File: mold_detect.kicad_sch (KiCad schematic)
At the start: 39 parts, among them J1 USB_C_Receptacle_USB2.0_14P, U1 SHT30-DIS, U2 TPL5010, U3 FT230XS, U4 W25Q128JVS, U5 ATmega328P-P, Y1 4MHz

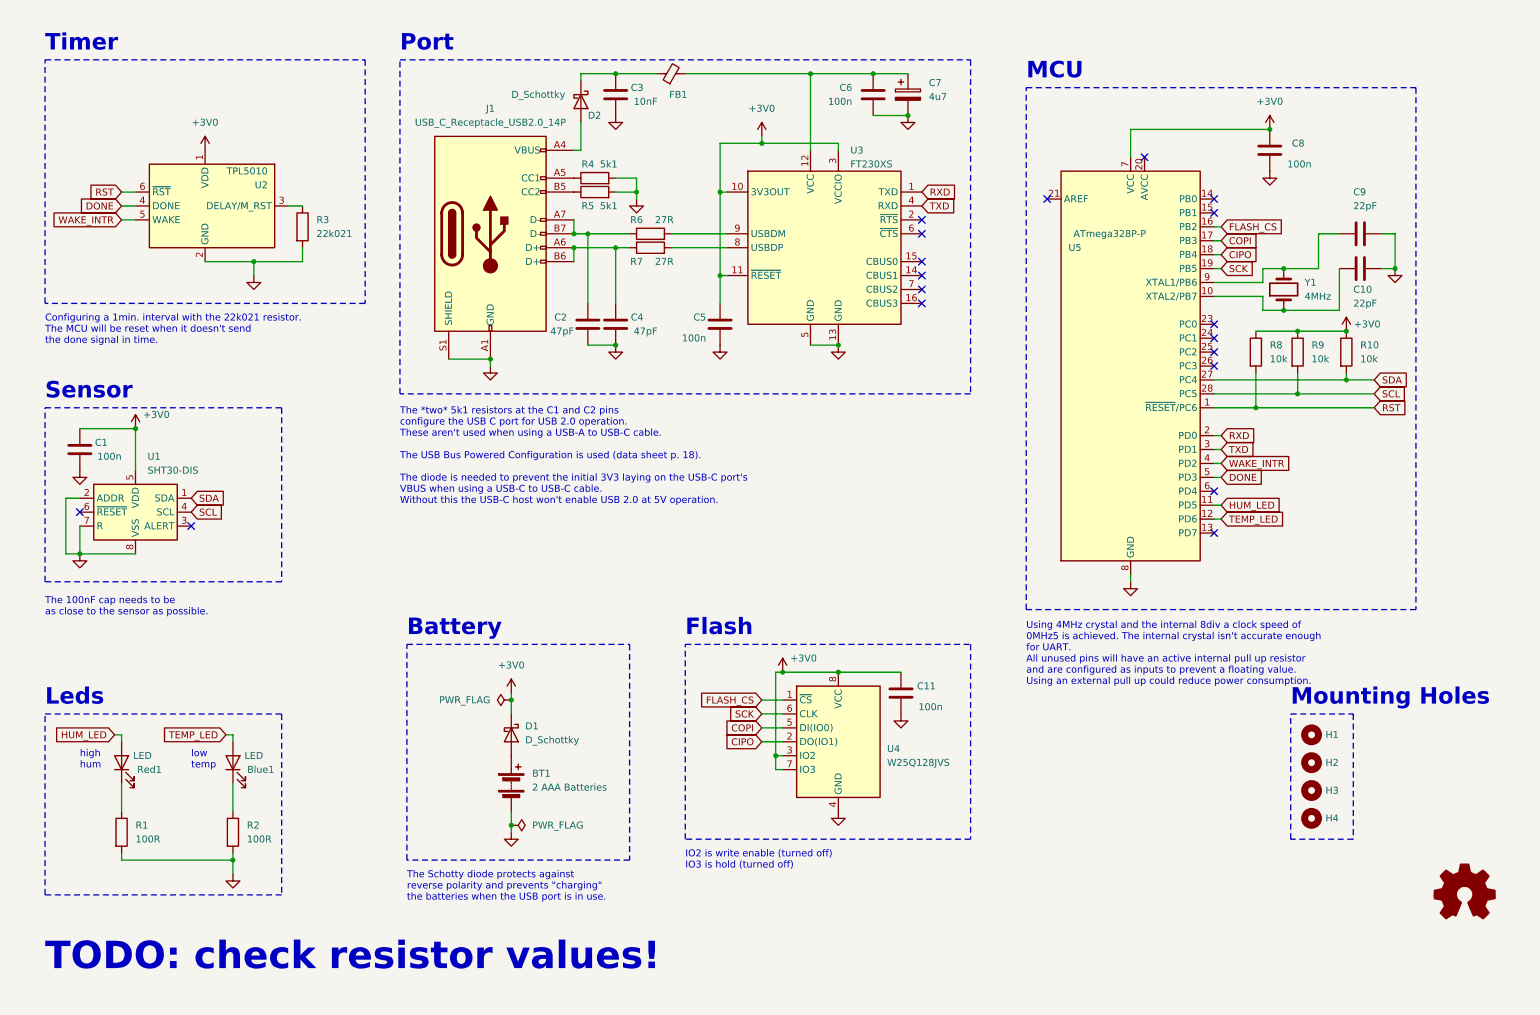
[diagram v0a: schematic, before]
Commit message: tpl5010 works!
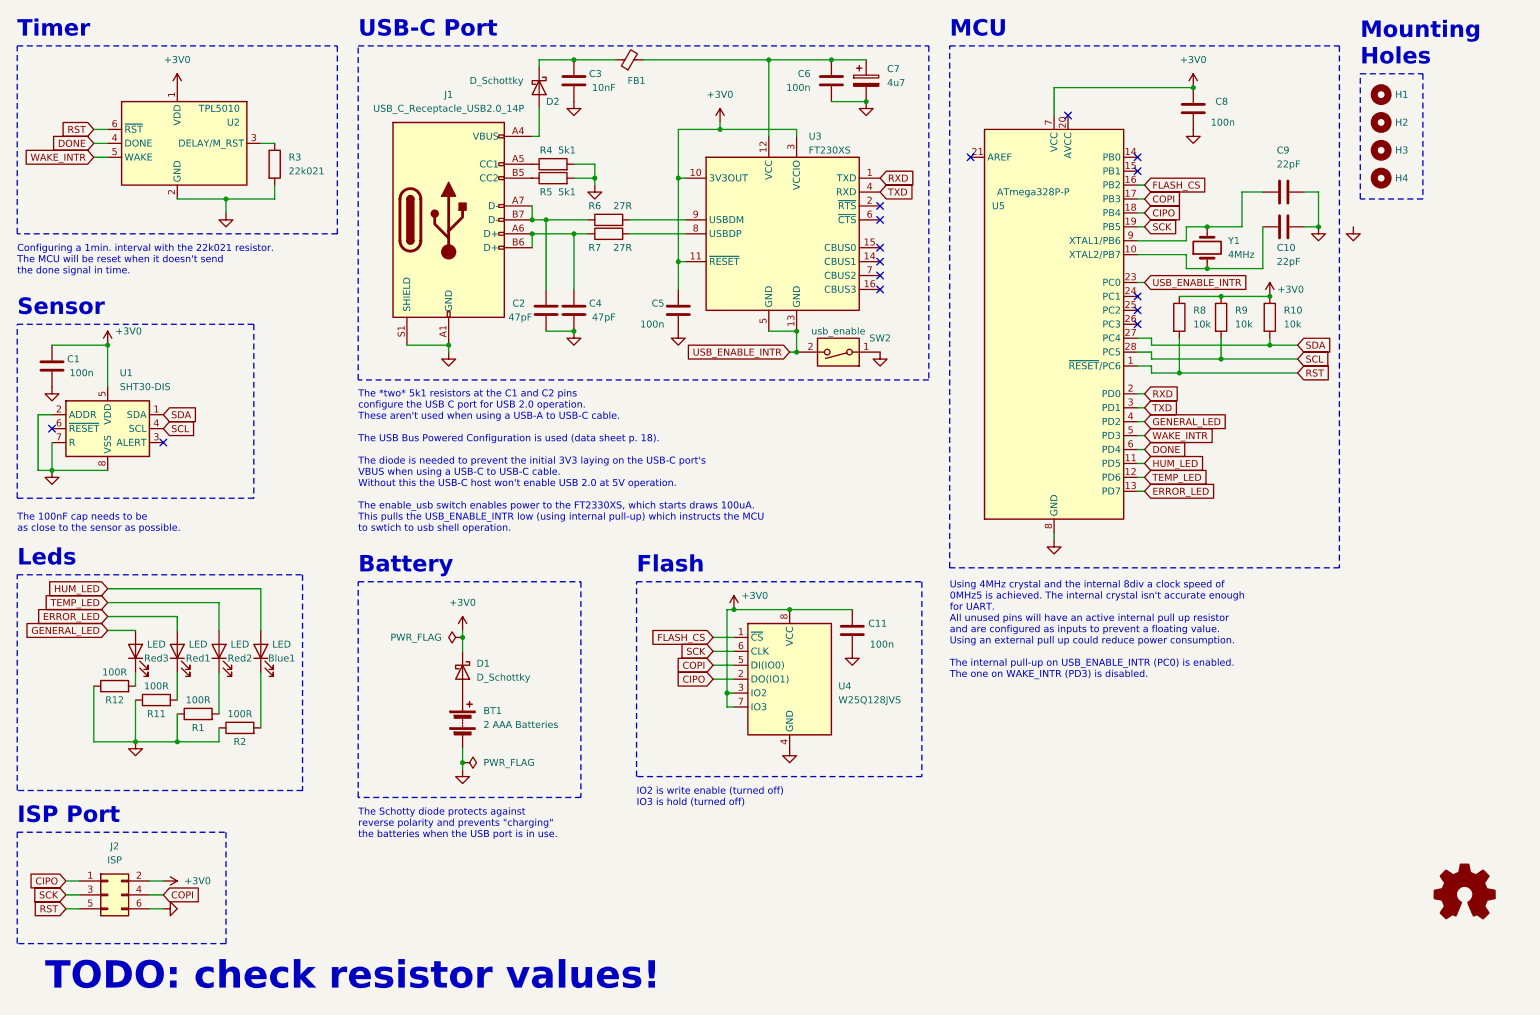
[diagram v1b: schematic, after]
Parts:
- added J2: ISP, Connector_IDC:IDC-Header_2x03_P2.54mm_Vertical, symbol Connector_Generic:Conn_02x03_Odd_Even
- added R11, R12: 100R, Resistor_SMD:R_0603_1608Metric_Pad0.98x0.95mm_HandSolder, symbol Device:R
- added Red2, Red3: LED, LED_THT:LED_D3.0mm, symbol Device:LED
- added SW2: usb_enable, symbol Switch:SW_DIP_x01
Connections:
- net +3V0: now also J2.2 (Pin_2)
- net CIPO: now also J2.1 (Pin_1)
- net COPI: now also J2.4 (Pin_4)
- net DONE: now also U5.6 (PD4); no longer U5.5 (PD3)
- net GND: now also R1.1, R2.1, J2.6 (Pin_6), R11.1, R12.1, SW2.1; no longer R1.2, R2.2, U3.13 (GND), U3.5 (GND)
- net HUM_LED: now also Blue1.2 (A); no longer Red1.2 (A)
- net RST: now also J2.5 (Pin_5)
- net SCK: now also J2.3 (Pin_3)
- net TEMP_LED: now also Red2.2 (A); no longer Blue1.2 (A)
- net WAKE_INTR: now also U5.5 (PD3); no longer U5.4 (PD2)
- net ERROR_LED: now reaches U5.13 (PD7)
- net ERROR_LED: now also Red1.2 (A)
- net USB_ENABLE_INTR: now reaches U5.23 (PC0)
- net USB_ENABLE_INTR: now also U3.13 (GND), U3.5 (GND), SW2.2
- net at Red1.1 (K): now also R11.2; no longer R1.1
- net at Blue1.1 (K): now also R2.2; no longer R2.1
- new net: R1.2, Red2.1 (K)
- new net: R12.2, Red3.1 (K)
- new net GENERAL_LED: Red3.2 (A), U5.4 (PD2)
- no-connect marks 18 -> 15
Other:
- note added: "ISP Port"
- note added: "The *two* 5k1 resistors at the C1 and C2 pins configure the USB C port for USB 2.0 operation. These aren't used when using a USB-A to USB-C cable. The USB Bus Powered Configuration is used (data sheet p. 18). The diode is needed to prevent the initial 3V3 laying on the USB-C port's VBUS when using a USB-C to USB-C cable. Without this the USB-C host won't enable USB 2.0 at 5V operation. The enable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"
- note added: "USB-C Port"
- note added: "Using 4MHz crystal and the internal 8div a clock speed of 0MHz5 is achieved. The internal crystal isn't accurate enough for UART. All unused pins will have an active internal pull up resistor and are configured as inputs to prevent a floating value. Using an external pull up could reduce power consumption. The internal pull-up on USB_ENABLE_INTR (PC0) is enabled. The one on WAKE_INTR (PD3) is dis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"
- note removed: "Port"
- note removed: "The *two* 5k1 resistors at the C1 and C2 pins configure the USB C port for USB 2.0 operation. These aren't used when using a USB-A to USB-C cable. The USB Bus Powered Configuration is used (data sheet p. 18). The diode is needed to prevent the initial 3V3 laying on the USB-C port's VBUS when using a USB-C to USB-C cable. Without this the USB-C host won't enable USB 2.0 at 5V operation."
- note removed: "Using 4MHz crystal and the internal 8div a clock speed of 0MHz5 is achieved. The internal crystal isn't accurate enough for UART. All unused pins will have an active internal pull up resistor and are configured as inputs to prevent a floating value. Using an external pull up could reduce power consumption."
- note removed: "high hum"
- note removed: "low temp"
- moved on the sheet: BT1, Blue1, C1, C10, C11, C2, C3, C4, C5, C6, C7, C8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
